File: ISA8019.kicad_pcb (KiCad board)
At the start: 2 copper layers, 104.1 x 71.9 mm, 58 parts, among them J1 Bus_ISA_8bit, J10 Extra Address Lines, J11 EPROM/SRAM Selection, J2 8P8C_Shielded, J4 Jumper mode, J5 PNP force, J6 BROM size and base address, J7 I/O base address, J8 Medium type, J9 IRQ Select, T1 13F-39MNL, U1 RTL8019AS, U2 AT93C46DN, U3 SST39SF040, Y1 20Mhz

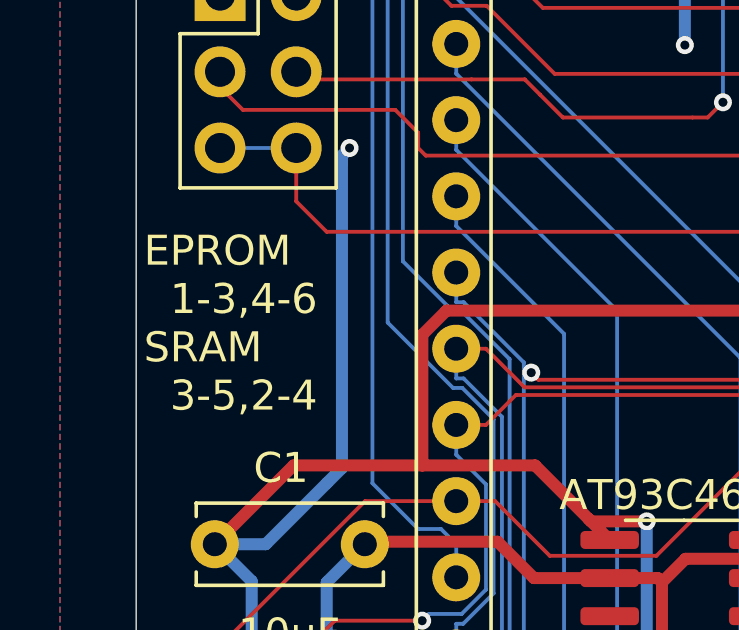
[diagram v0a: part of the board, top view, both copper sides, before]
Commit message: Add Revision 2.4
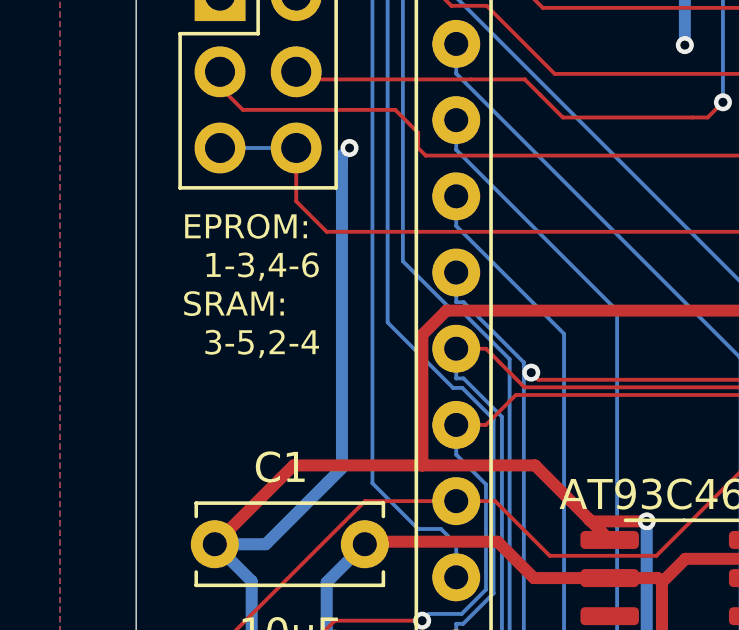
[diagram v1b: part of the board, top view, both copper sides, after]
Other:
- board text added: "EPROM: 1-3,4-6 SRAM: 3-5,2-4"
- board text removed: "EPROM 1-3,4-6 SRAM 3-5,2-4"
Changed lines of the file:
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@@
       (drillshape 0)
       (scaleselection 1)
-      (outputdirectory "gerbers/Rev_2.3")
+      (outputdirectory "gerbers/Rev_2.4")
     )
   )
@@
     (effects (font (size 1 1) (thickness 0.15)))
   )
-  (gr_text "EPROM\n  1-3,4-6\nSRAM\n  3-5,2-4" (at 79.308 94.784) (layer "F.SilkS")
-    (effects (font (size 1 1) (thickness 0.25)) (justify left))
+  (gr_text "EPROM:\n  1-3,4-6\nSRAM:\n  3-5,2-4" (at 80.578 93.514) (layer "F.SilkS")
+    (effects (font (size 0.8 0.8) (thickness 0.15)) (justify left))
   )
   (gr_text "3 2 1 0" (at 86.674 57.573) (layer "F.SilkS")
